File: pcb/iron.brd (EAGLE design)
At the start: 8 x 26 mm, 25 parts, among them IC1 AT24CS04-SOT23, IC2 TS507CLT, IC3 AD7995, IC4 ESDA6V1SC5, X1 LUMBERG_KLB_4

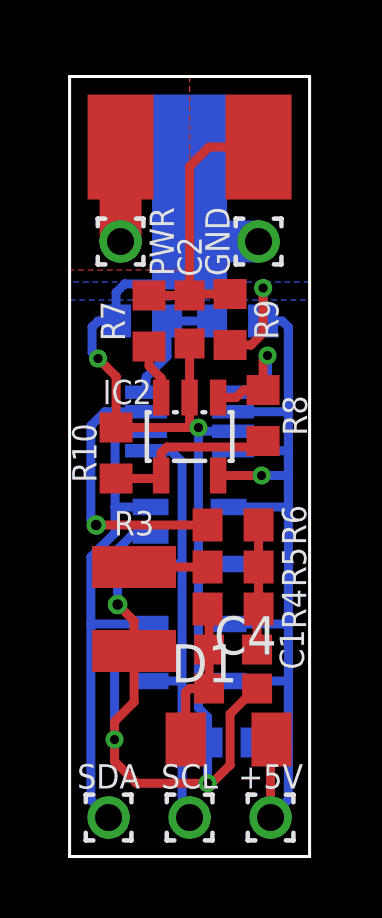
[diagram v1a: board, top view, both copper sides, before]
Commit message: boms reworked
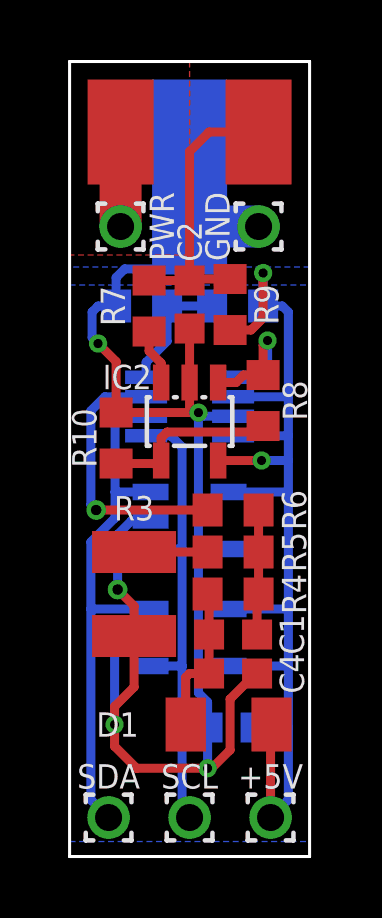
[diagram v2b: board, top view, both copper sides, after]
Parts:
- moved D1 0.50 mm to (5.30, 4.40)
- moved C1 0.50 mm to (5.45, 7.40)
- moved C2 0.50 mm to (4.00, 18.4)
- moved C3 0.50 mm to (5.40, 4.30)
- moved C4 0.50 mm to (5.45, 6.10)
- moved GND 0.50 mm to (6.30, 21.0)
- moved IC1 0.50 mm to (4.00, 11.2)
- moved IC2 0.50 mm to (4.00, 14.5)
- moved IC3 0.50 mm to (4.00, 15.0)
- moved IC4 0.50 mm to (4.00, 7.30)
- moved PWR 0.50 mm to (1.70, 21.0)
- moved R1 0.50 mm to (5.60, 18.4)
- moved R10 0.50 mm to (1.55, 13.9)
- moved R2 0.50 mm to (2.40, 18.4)
- moved R3 0.50 mm to (2.15, 8.75)
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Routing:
- net +5V: track 37.1 -> 38.1 mm
- net SDA: track 17.5 -> 18.0 mm
- net SCL: track 15.4 -> 15.9 mm
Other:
- board size 8 x 26 mm -> 8 x 26.5 mm
